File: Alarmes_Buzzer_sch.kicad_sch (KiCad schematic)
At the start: 29 parts, among them Q58 2N7000, Q59 2N7000, Q60 2N7000, Q61 2N7000, Q62 2N7000, Q63 2N7000

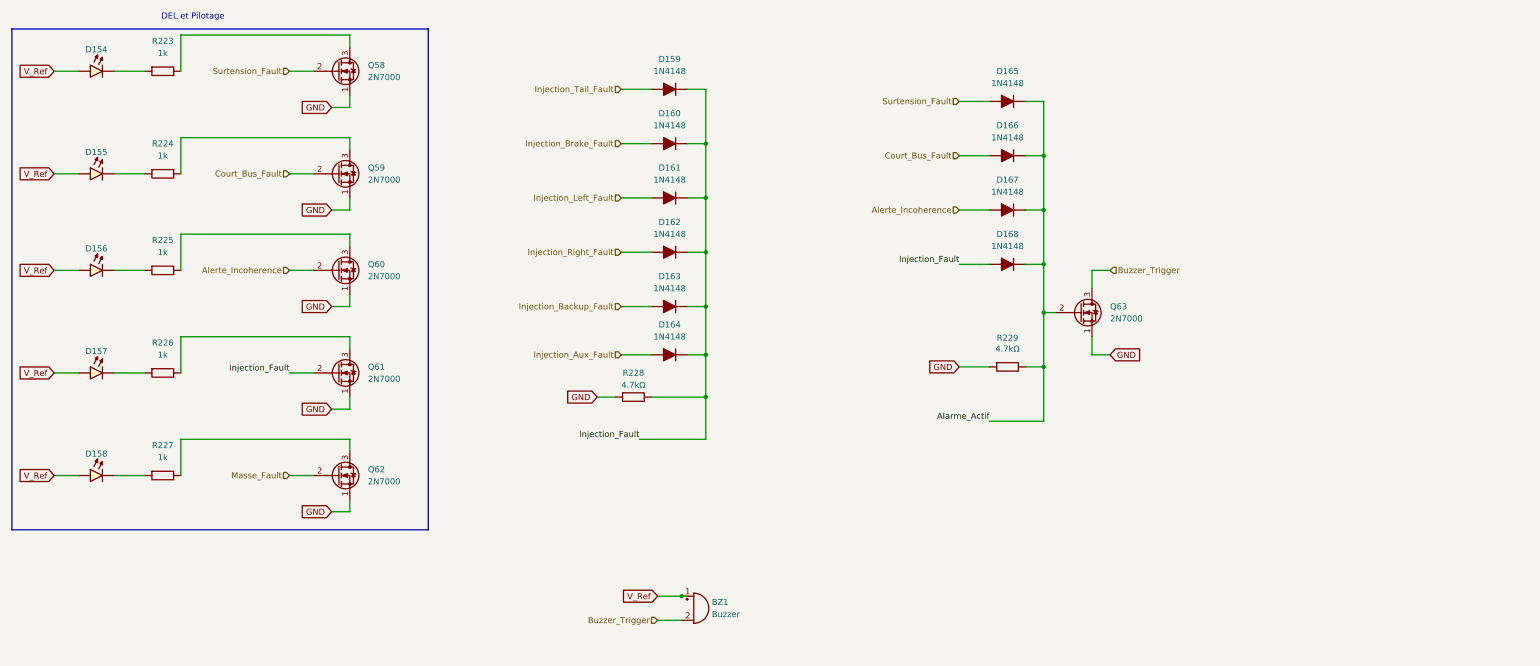
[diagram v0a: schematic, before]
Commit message: Add files via upload
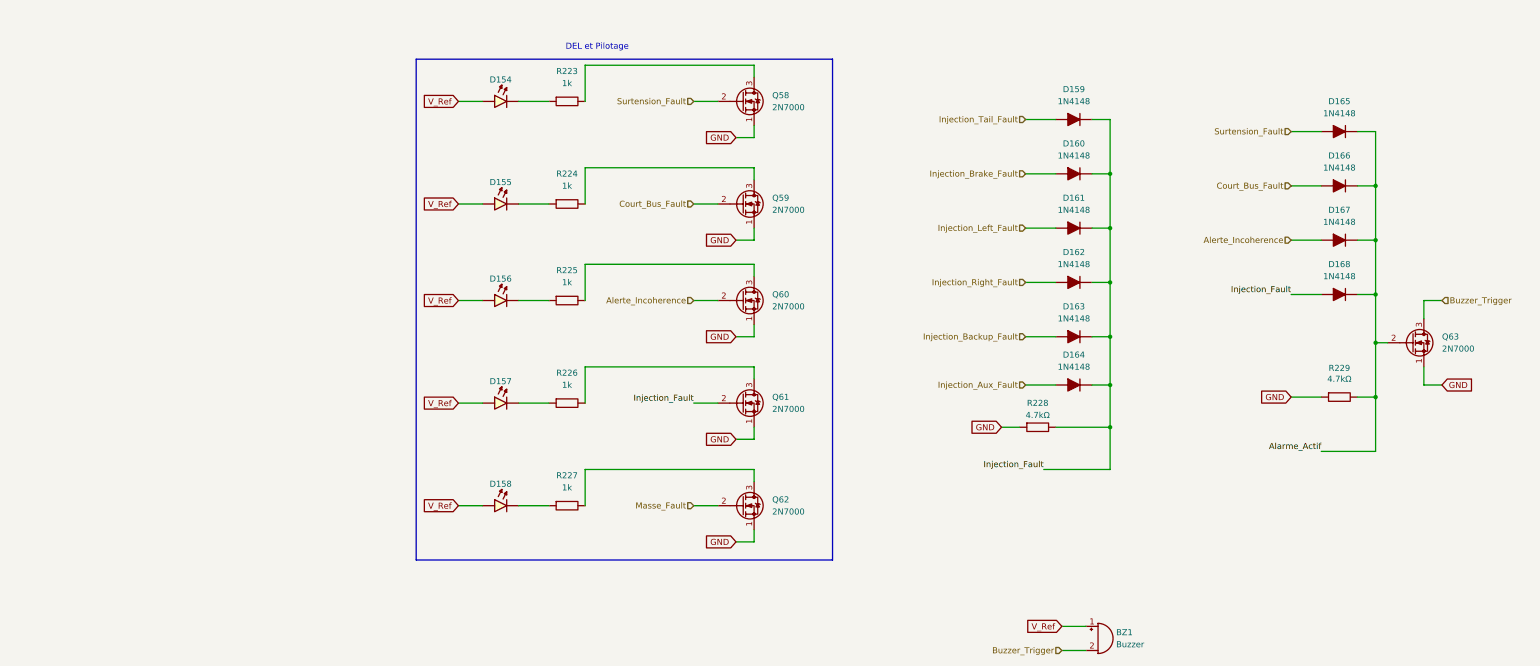
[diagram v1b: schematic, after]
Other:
- moved on the sheet: BZ1, D154, D155, D156, D157, D158, D159, D160, D161, D162, D163, D164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
